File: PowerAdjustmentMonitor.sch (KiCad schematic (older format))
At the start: 18 parts, among them U5 LM317K, U6 7805, U7 7805, U8 LM317K, U9 LM324

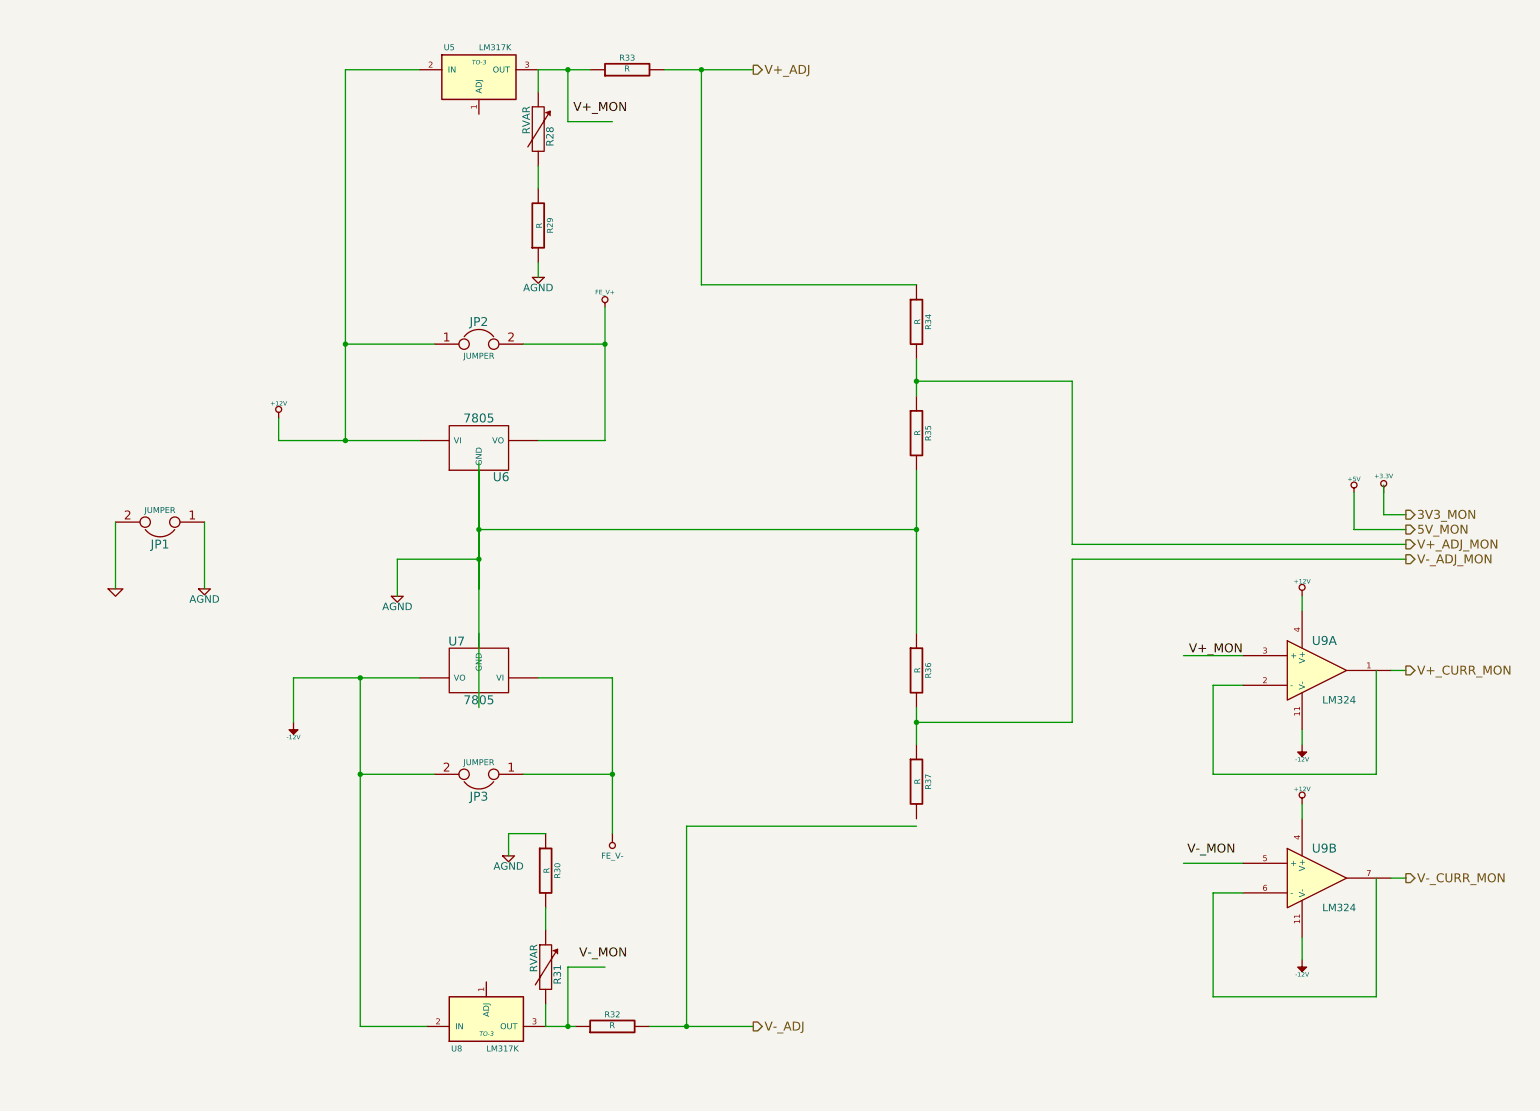
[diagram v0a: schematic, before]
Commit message: 5.10 Video 1/2 Associating and Placing the Power Modification Module
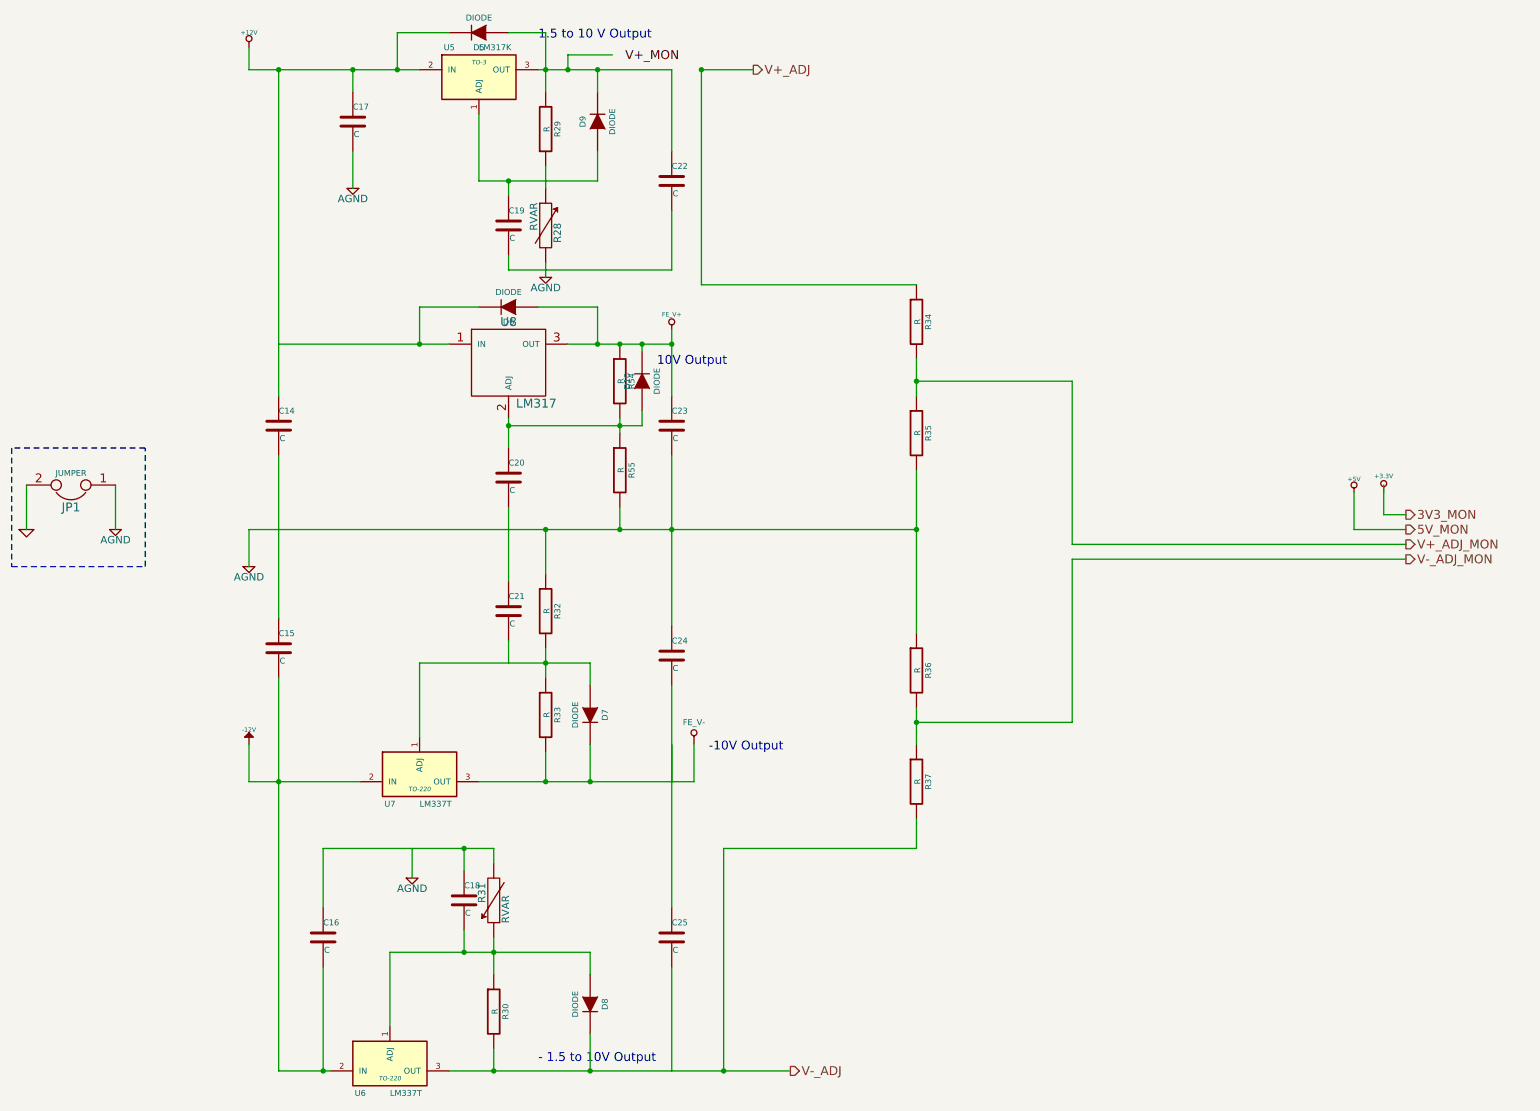
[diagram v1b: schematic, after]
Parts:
- removed JP2, JP3: JUMPER, symbol JUMPER
- removed U6, U7: 7805, symbol 7805
- removed U8: LM317K, TO-3, symbol LM317K
- removed U9: LM324, symbol LM324
- added C14, C15, C16, C17, C18, C19, C20, C21, C22, C23, C24, C25: C, ~, symbol C
- added D10, D5, D6, D7, D8, D9: DIODE, ~, symbol DIODE
- added R54, R55: R, ~, symbol R
- added U6, U7: LM337T, TO-220, symbol LM337T
- added U8: LM317, ~, symbol LM317
- R30, R32, R33: footprint (none) -> ~
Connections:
- net labels removed: V+_CURR_MON, V-_CURR_MON, V-_MON
- wire segments 71 -> 93
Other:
- note added: "- 1.5 to 10V Output"
- note added: "-10V Output"
- note added: "1.5 to 10 V Output"
- note added: "10V Output"
- moved on the sheet: JP1, R28, R29
